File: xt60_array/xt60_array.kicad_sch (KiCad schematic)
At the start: 1 part, among them J1 XT60_INPUT

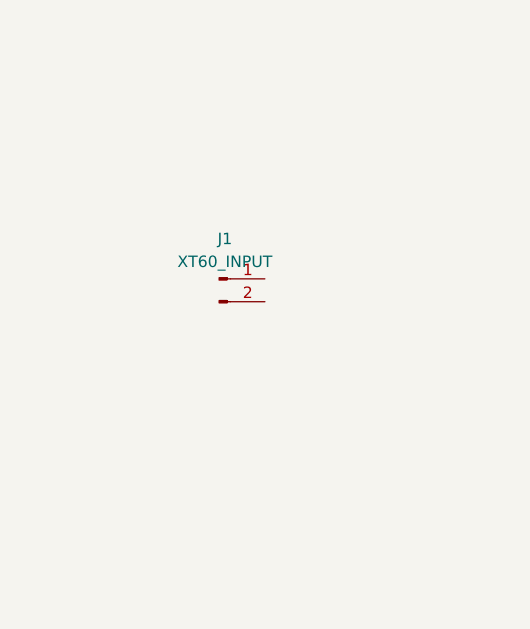
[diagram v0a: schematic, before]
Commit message: Finished schematic
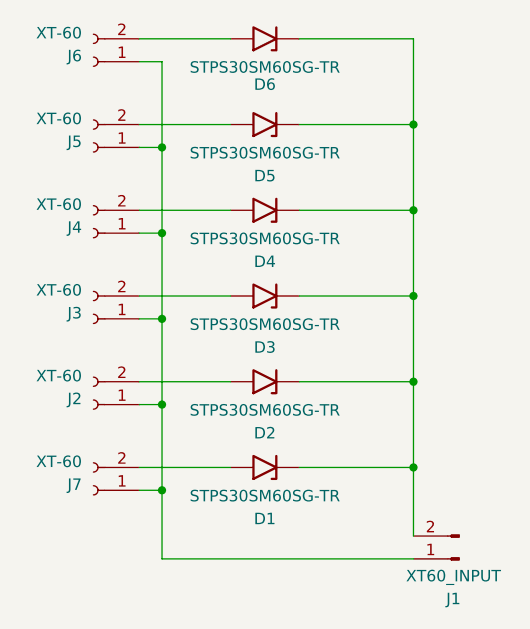
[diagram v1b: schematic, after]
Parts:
- added D1, D2, D3, D4, D5, D6: STPS30SM60SG-TR, Matt:TO-263-2_TabPin1_Alt, symbol Diode:1.5KExxA
- added J2, J3, J4, J5, J6, J7: XT-60, Connector_AMASS:AMASS_XT60-M_1x02_P7.20mm_Vertical, symbol Connector:Conn_01x02_Socket
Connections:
- net at J1.1 (Pin_1): now also J2.1 (Pin_1), J3.1 (Pin_1), J4.1 (Pin_1), J5.1 (Pin_1), J6.1 (Pin_1), J7.1 (Pin_1)
- net at J1.2 (Pin_2): now also D1.1 (A1), D2.1 (A1), D3.1 (A1), D4.1 (A1), D5.1 (A1), D6.1 (A1)
- new net: D4.2 (A2), J4.2 (Pin_2)
- new net: D2.2 (A2), J2.2 (Pin_2)
- new net: D1.2 (A2), J7.2 (Pin_2)
- new net: D5.2 (A2), J5.2 (Pin_2)
- new net: D3.2 (A2), J3.2 (Pin_2)
- new net: D6.2 (A2), J6.2 (Pin_2)
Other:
- moved on the sheet: J1
